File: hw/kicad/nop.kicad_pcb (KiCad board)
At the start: 2 copper layers, 203.2 x 165.1 mm, 90 parts, among them J1 PS/2, J2 +5V, J3 SD Breakout, J4 Reset, J5 TV, J6 RS232, Q1 2N4401, U1 W65C02S, U10 ATF16V8, U13 74HCT00, U15 74HCT00, U16 74HCT574, U17 74HCT574, U18 74HCT574, U19 74HCT04, U2 TMS9118A, U20 LM386, U21 74HCT595, U22 74HCT595, U23 74HCT14, U24 MAX232, U3 W65C22S, U4 16550, U5 SN76489AN, U6 62256, U7 62256, U8 2864, U9 62256, Y1 1Mhz, Y3 11.0592Mhz, Y4 10.738635Mhz

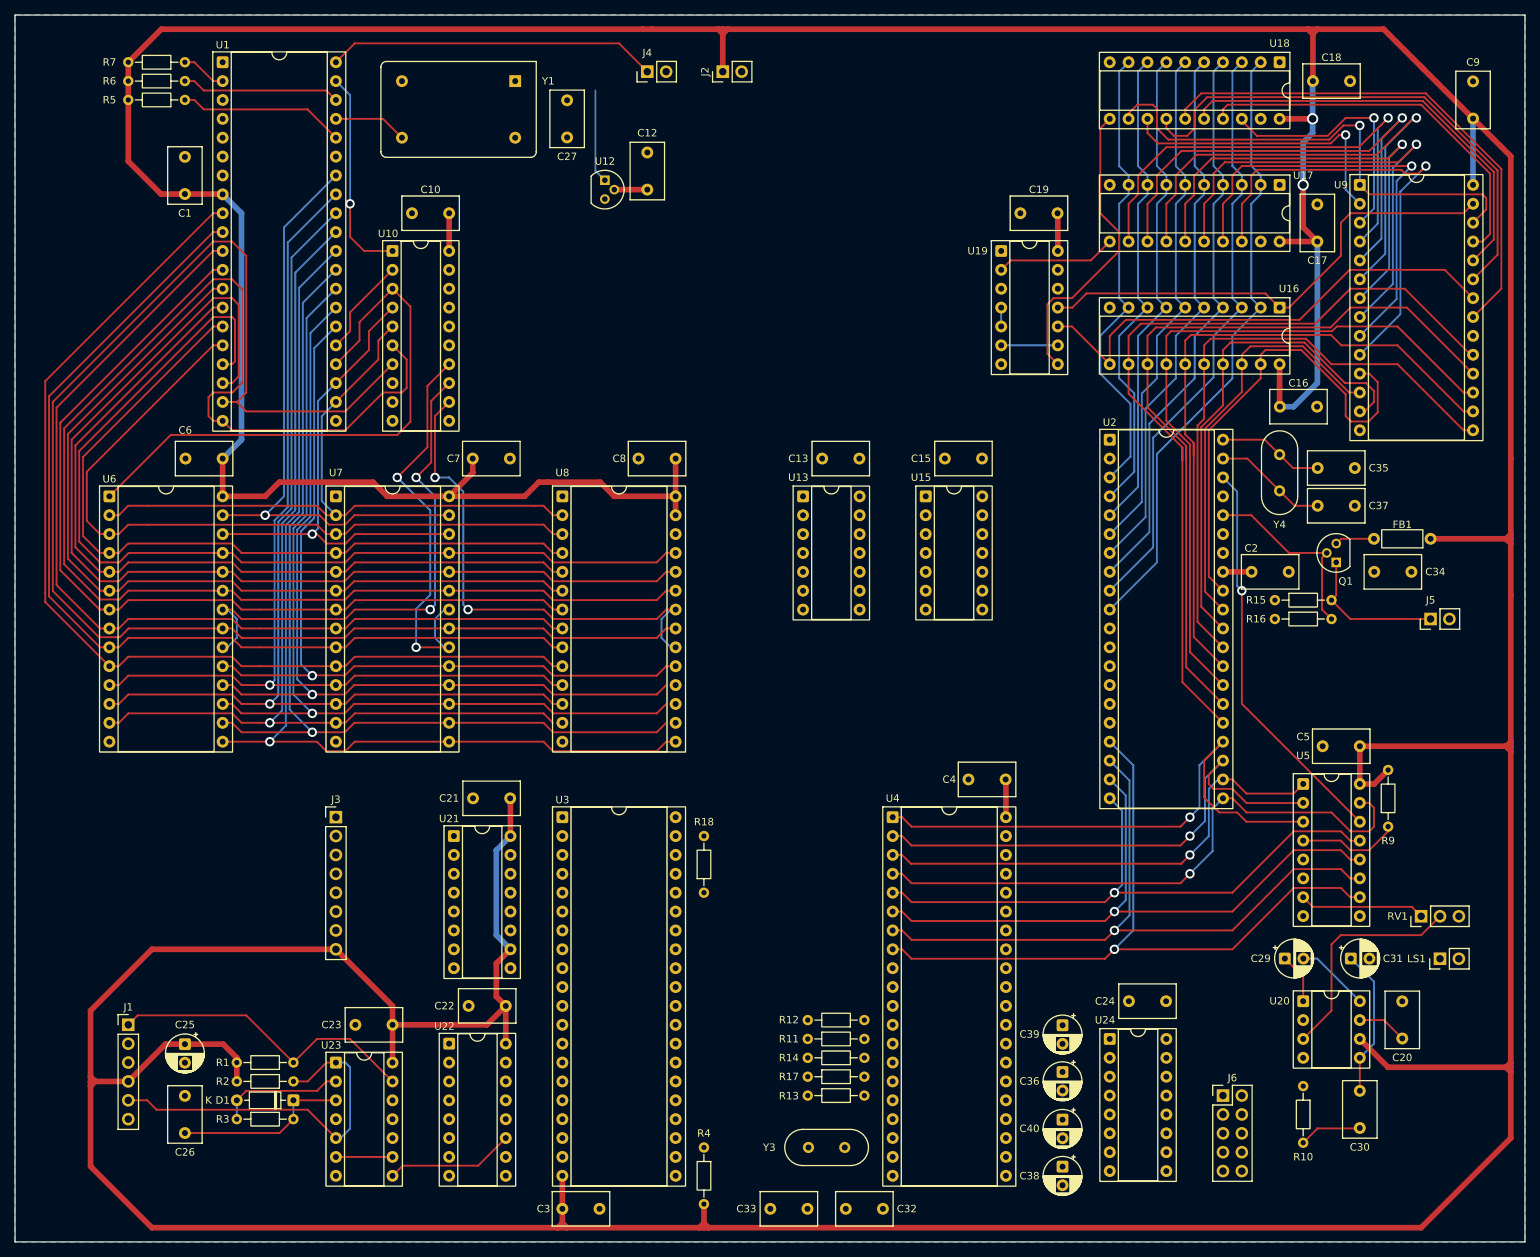
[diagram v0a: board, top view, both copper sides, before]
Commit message: hw: complete layout
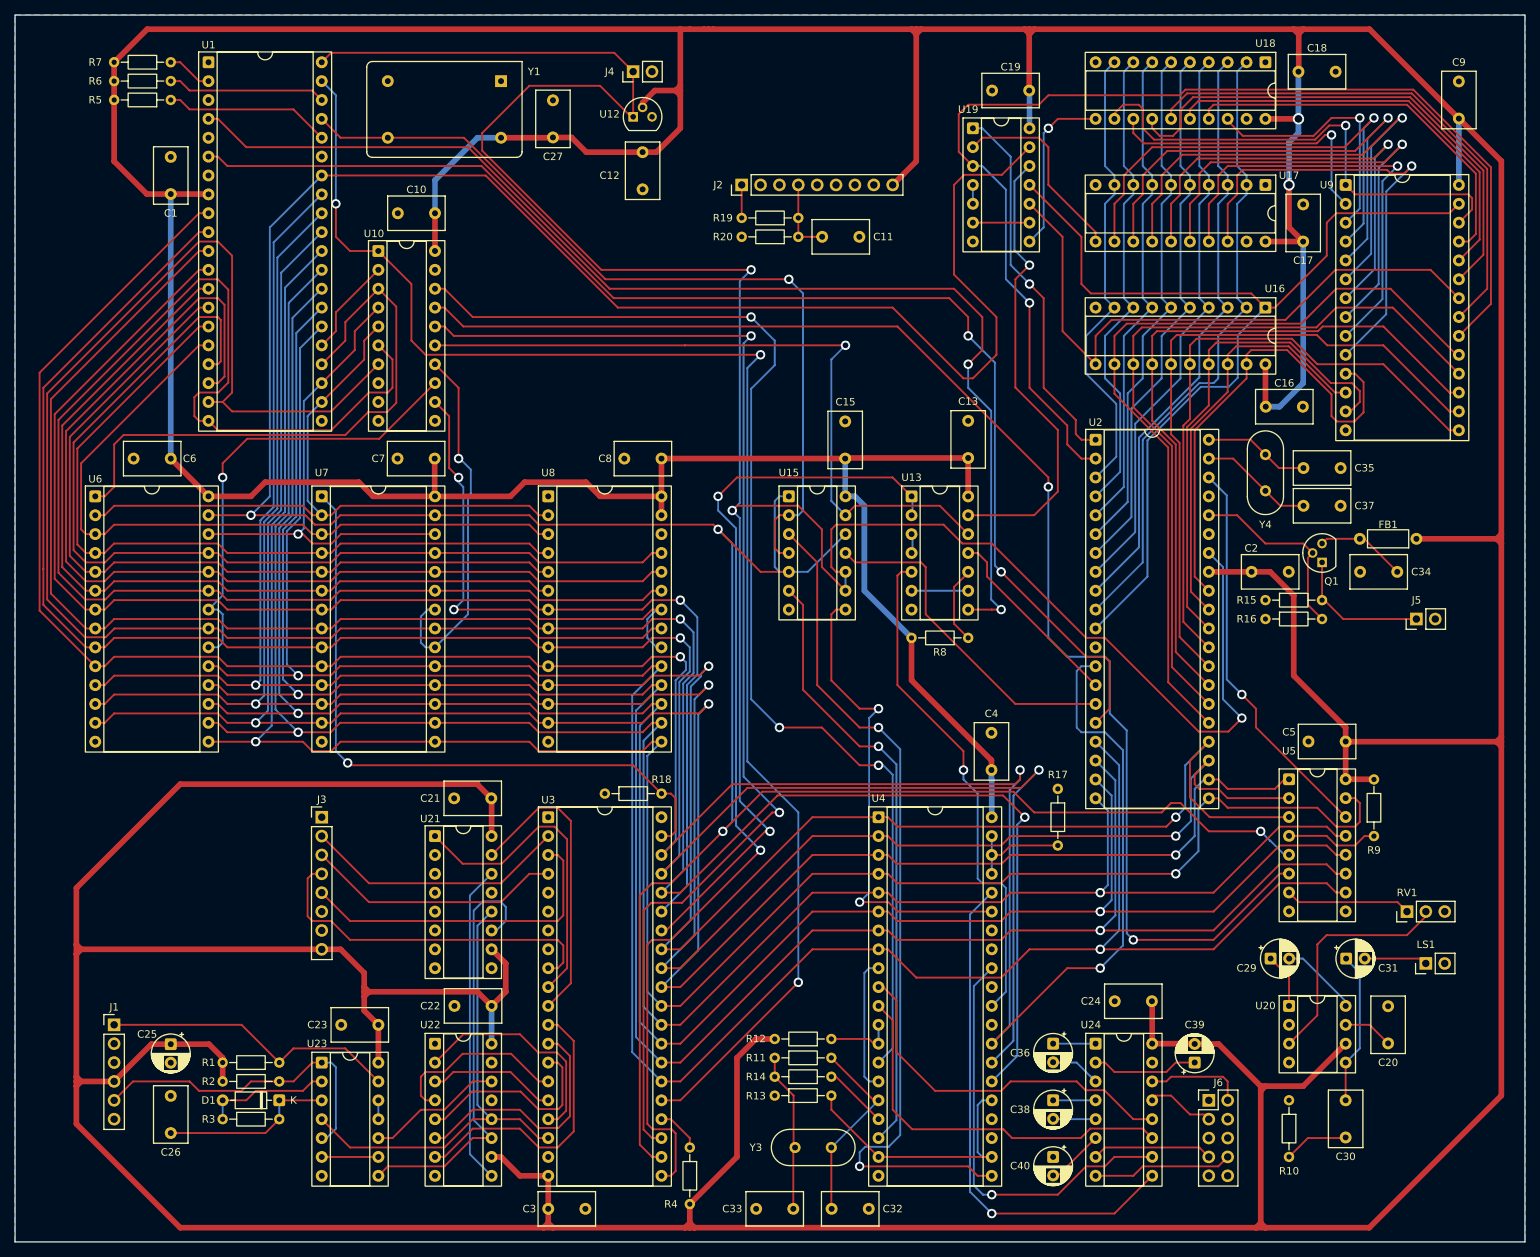
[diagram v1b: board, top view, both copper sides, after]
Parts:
- added C11: 0.1uF, Capacitor_THT:C_Disc_D7.5mm_W4.4mm_P5.00mm, F.Cu at (125.7, 41.9)
- added R19: 91K, Resistor_THT:R_Axial_DIN0204_L3.6mm_D1.6mm_P7.62mm_Horizontal, F.Cu at (117.5, 39.4)
- added R20: 27K, Resistor_THT:R_Axial_DIN0204_L3.6mm_D1.6mm_P7.62mm_Horizontal, F.Cu at (117.5, 41.9)
- added R8: 10K, Resistor_THT:R_Axial_DIN0204_L3.6mm_D1.6mm_P7.62mm_Horizontal, F.Cu at (140.3, 95.9)
- J2: value +5V -> LM73100 Breakout; footprint Connector_PinHeader_2.54mm:PinHeader_1x02_P2.54mm_Vertical -> Connector_PinHeader_2.54mm:PinHeader_1x09_P2.54mm_Vertical
- U12: value ~ -> DS1813
- moved R17 51.3 mm to (152.4, 116.2), turned to -90 degrees
- moved R18 18.9 mm to (91.4, 116.8), turned to 0 degrees
- moved C39 18.5 mm to (170.8, 153.0), turned to 90 degrees
- moved U15 18.4 mm to (116.2, 76.8)
- moved C15 18.4 mm to (123.8, 71.8), turned to 90 degrees
- moved C19 16.9 mm to (148.6, 22.2)
- moved U19 16.9 mm to (141.0, 27.3)
- moved J2 15.5 mm to (109.9, 34.9)
- moved C13 14.6 mm to (140.3, 71.7), turned to 90 degrees
- moved U13 14.6 mm to (132.7, 76.8)
- moved U12 9.34 mm to (95.2, 25.8), turned to 0 degrees
- moved C38 9.02 mm to (151.8, 158.1)
- moved C6 6.99 mm to (33.0, 71.8)
- moved C40 5.17 mm to (151.8, 165.7)
- moved R12 5.12 mm to (121.9, 149.9)
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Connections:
- J2 pad 1: +5V -> Net-(J2-Vin)
- U13 pad 10: Net-(U13-Pad10) -> ~{i2}
- U13 pad 4: i1 -> Net-(U13-Pad3)
- U13 pad 5: +5V -> i1
- U13 pad 6: Net-(U13-Pad10) -> Net-(U13-Pad6)
- U13 pad 9: Net-(U13-Pad3) -> Net-(U13-Pad6)
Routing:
- net r/~{w}: track 81.8 -> 473.6 mm, vias 1 -> 4
- net +5V: track 1024.3 -> 1369.4 mm
- net ~{res}: track 57.1 -> 344.4 mm, vias 0 -> 4
- net a0: track 138.2 -> 343.4 mm, vias 0 -> 3
- net ~{dev2}: track 0.01 -> 186.6 mm, vias 0 -> 2
- net ~{nmi}: track 0.00 -> 176.0 mm, vias 0 -> 2
- net phi2: track 28.2 -> 203.0 mm, vias 1 -> 3
- net ~{dev1}: track 0.00 -> 165.7 mm, vias 0 -> 2
- net ~{irq}: track 0.00 -> 161.5 mm, vias 0 -> 2
- net ~{dev3}: track 0.00 -> 161.0 mm, vias 0 -> 3
- net Net-(U2-~{CAS}): track 0.00 -> 157.6 mm, vias 0 -> 1
- net /a1: track 134.2 -> 284.0 mm, vias 0 -> 2
- net /a2: track 127.6 -> 277.2 mm, vias 0 -> 2
- net ~{i0}: track 0.00 -> 137.0 mm, vias 0 -> 2
- net Net-(U4-~{RD}): track 0.00 -> 115.2 mm, vias 0 -> 2
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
